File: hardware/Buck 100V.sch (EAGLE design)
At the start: 31 parts, among them M1 SI3430DV, M2 SI5435BDC, Q1 FMMT625, Q2 FMMT723, U1 LT3756EMSE

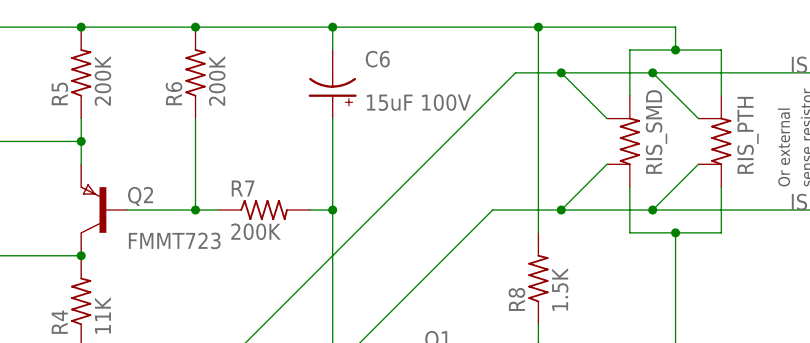
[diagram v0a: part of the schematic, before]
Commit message: Very rough initial board layout. Can now safely say that the board will be smaller than 2 inches by 3 inches.
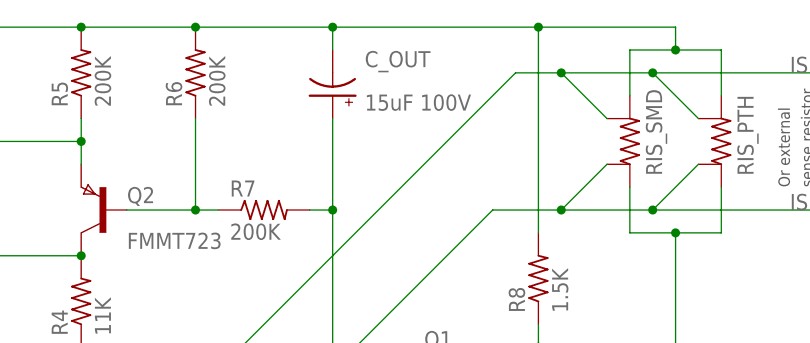
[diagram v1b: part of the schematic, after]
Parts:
- renumbered C6 to C_OUT
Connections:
- net N$12 renamed N_BUCK
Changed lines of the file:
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@@
 <part name="JH" library="con-lstb" deviceset="MA06-1" device=""/>
 <part name="JL" library="con-lstb" deviceset="MA08-1" device=""/>
-<part name="C6" library="rcl" deviceset="CPOL-US" device="E2,5-6E" value="15uF 100V"/>
+<part name="C_OUT" library="rcl" deviceset="CPOL-US" device="E2,5-6E" value="15uF 100V"/>
 <part name="RIS_SMD" library="LED-drivers" deviceset="R-KELVIN" device="R2512"/>
 <part name="RIS_PTH" library="LED-drivers" deviceset="R-KELVIN" device="0204/7"/>
@@
 <instance part="JH" gate="1" x="182.88" y="50.8" rot="R180"/>
 <instance part="JL" gate="1" x="182.88" y="22.86" rot="R180"/>
-<instance part="C6" gate="G$1" x="66.04" y="55.88" smashed="yes" rot="R180">
+<instance part="C_OUT" gate="G$1" x="66.04" y="55.88" smashed="yes" rot="R180">
 <attribute name="NAME" x="69.596" y="59.055" size="1.778" layer="95"/>
 <attribute name="VALUE" x="69.596" y="54.229" size="1.778" layer="96"/>
@@
 <wire x1="-58.42" y1="58.42" x2="-58.42" y2="63.5" width="0.1524" layer="91"/>
 <junction x="-58.42" y="63.5"/>
-<pinref part="C6" gate="G$1" pin="-"/>
+<pinref part="C_OUT" gate="G$1" pin="-"/>
 <pinref part="RIS_PTH" gate="G$1" pin="2"/>
 <wire x1="109.22" y1="55.88" x2="109.22" y2="60.96" width="0.1524" layer="91"/>
@@
 <wire x1="66.04" y1="53.34" x2="66.04" y2="43.18" width="0.1524" layer="91"/>
 <junction x="66.04" y="43.18"/>
-<pinref part="C6" gate="G$1" pin="+"/>
+<pinref part="C_OUT" gate="G$1" pin="+"/>
 </segment>
 <segment>
@@
 </segment>
 </net>
-<net name="N$12" class="0">
+<net name="N_BUCK" class="0">
 <segment>
 <pinref part="L1" gate="G$1" pin="1"/>
